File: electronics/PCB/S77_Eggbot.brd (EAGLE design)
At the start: 95.2 x 68.2 mm, 5 parts, among them U1 CR_LM2596, U2 S2_MINI, U3 CARRIER_A4988, U4 CARRIER_A4988, X1 POLLIN_JACK_A

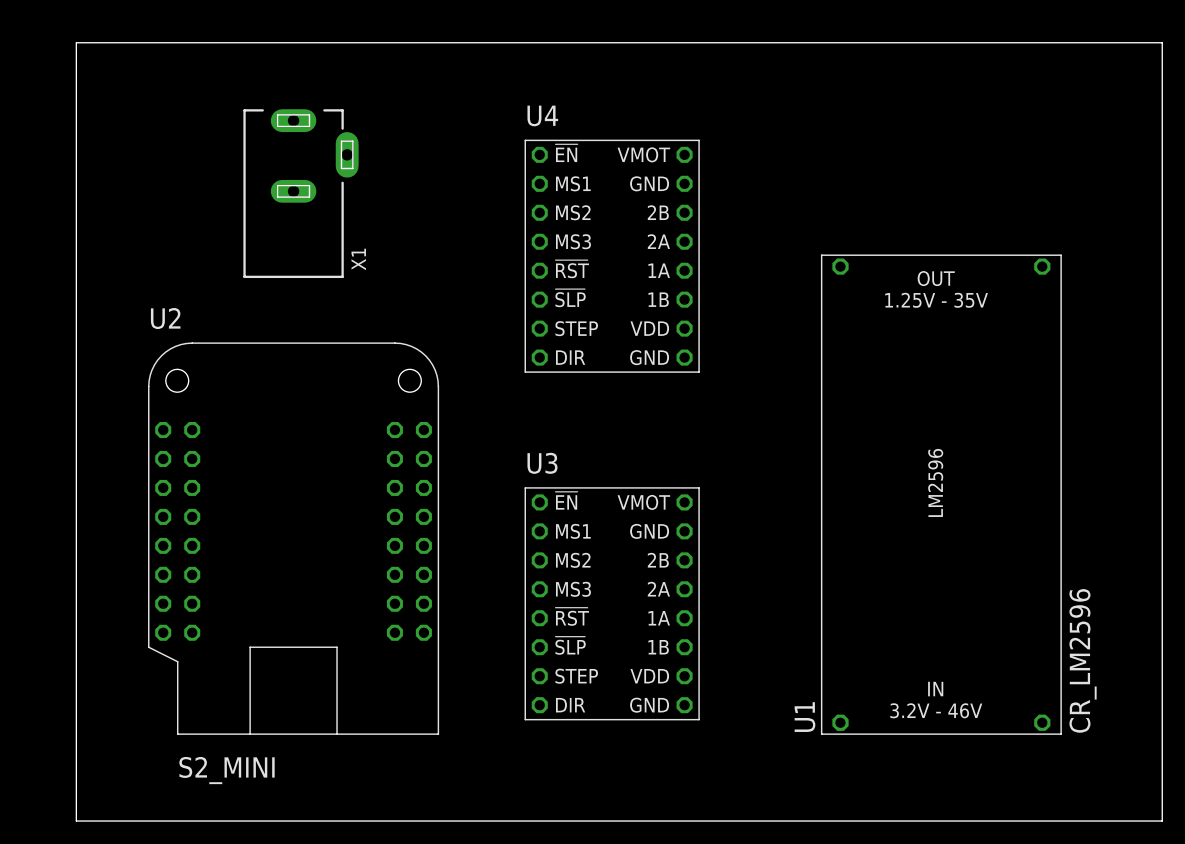
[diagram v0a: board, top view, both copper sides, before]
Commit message: WIP: fix board dimension and place components
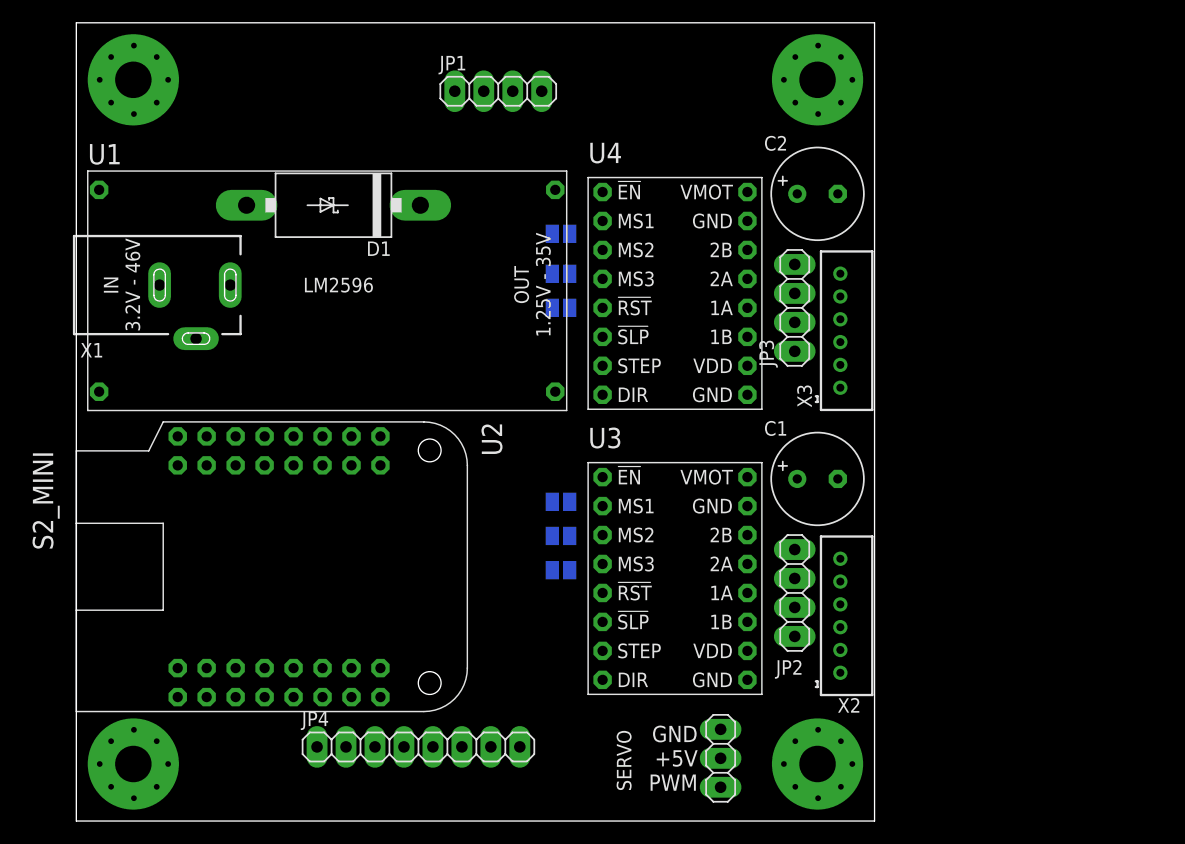
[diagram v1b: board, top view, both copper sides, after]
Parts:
- added C1, C2: 100µF/35V/0R056, rcl:E3,5-8
- added D1: 1N5822, lib_s77_eggbot:DO201T15
- added JP1, JP2, JP3: (no value), pinhead:1X04
- added JP4: (no value), pinhead:1X08
- added SERVO: (no value), pinhead:1X03
- added SJ1, SJ2, SJ3, SJ4, SJ5, SJ6: (no value), jumper:SJ
- added X2, X3: B6B-PH, lib_s77_eggbot:B6B-PH
- X1: value POLLIN_JACK_A -> PWR
- moved U1 90.0 mm to (1.00, 36.0), turned to 0 degrees
- moved U2 28.1 mm to (0.00, 35.0), turned to 270 degrees
- moved X1 14.3 mm to (10.5, 47.0), turned to 270 degrees
- moved U4 6.40 mm to (52.5, 45.0)
- moved U3 5.94 mm to (52.5, 20.0)
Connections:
- new net +5V: JP1.2, U1.4
- new net N$10: JP3.4, U4.14, X3.6
- new net N$11: SJ1.2, U3.2
- new net N$12: SJ2.2, U3.3
- new net N$13: SJ3.2, U3.4
- new net N$14: U3.1
- new net N$15: U3.8
- new net N$16: U3.7
- new net N$17: SJ4.2, U4.2
- new net N$18: SJ5.2, U4.3
- new net N$19: SJ6.2, U4.4
- new net N$2: JP2.1, U3.11, X2.1
- new net N$3: D1.A, X1.1
- new net N$4: JP2.2, U3.12, X2.2
- new net N$5: JP2.3, U3.13, X2.4
- new net N$6: JP2.4, U3.14, X2.6
- new net N$7: JP3.1, U4.11, X3.1
- new net N$8: JP3.2, U4.12, X3.2
- new net N$9: JP3.3, U4.13, X3.4
- net +3V3: now also JP1.3, SJ1.1, SJ2.1, SJ3.1, SJ4.1, SJ5.1, SJ6.1, U3.10, U3.5, U3.6, U4.5, U4.6
- net GND: now also C1.-, C2.-, JP1.4, X1.2
- net VDD: no longer U3.10
- net VMOT: now also C1.+, C2.+, D1.C, JP1.1, U1.1
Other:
- board size 95.2 x 68.2 mm -> 70 x 70 mm
- board text added: "GND +5V PWM"
